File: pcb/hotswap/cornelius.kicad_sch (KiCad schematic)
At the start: 116 parts, among them J1 AVR-ISP-6, SW1 SW_Push, U1 ATmega32U4-M, U2 PRTR5V0U2X, Y1 16MHz

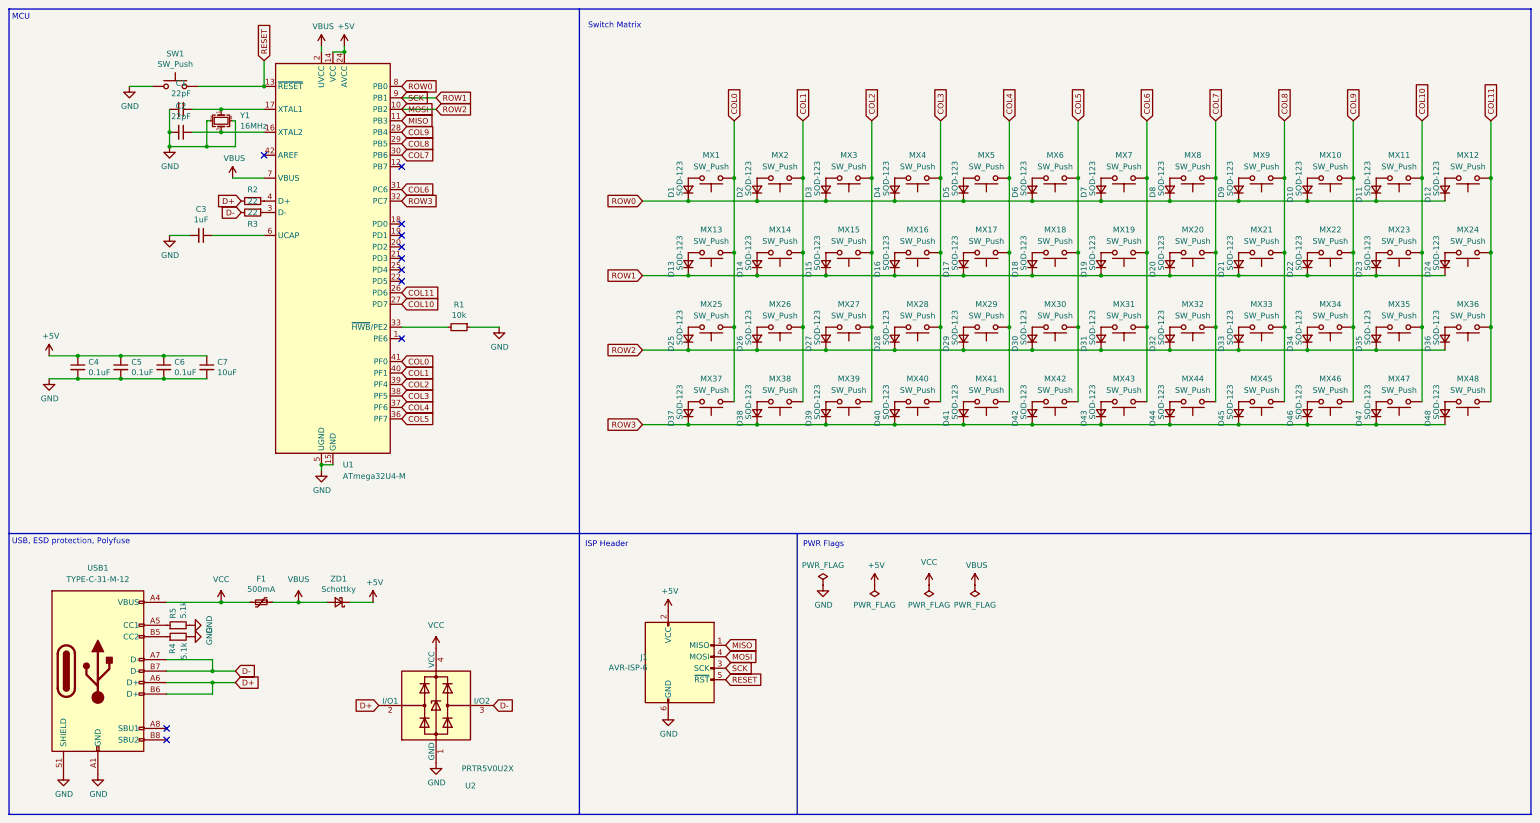
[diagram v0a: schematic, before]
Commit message: Add solder pcb
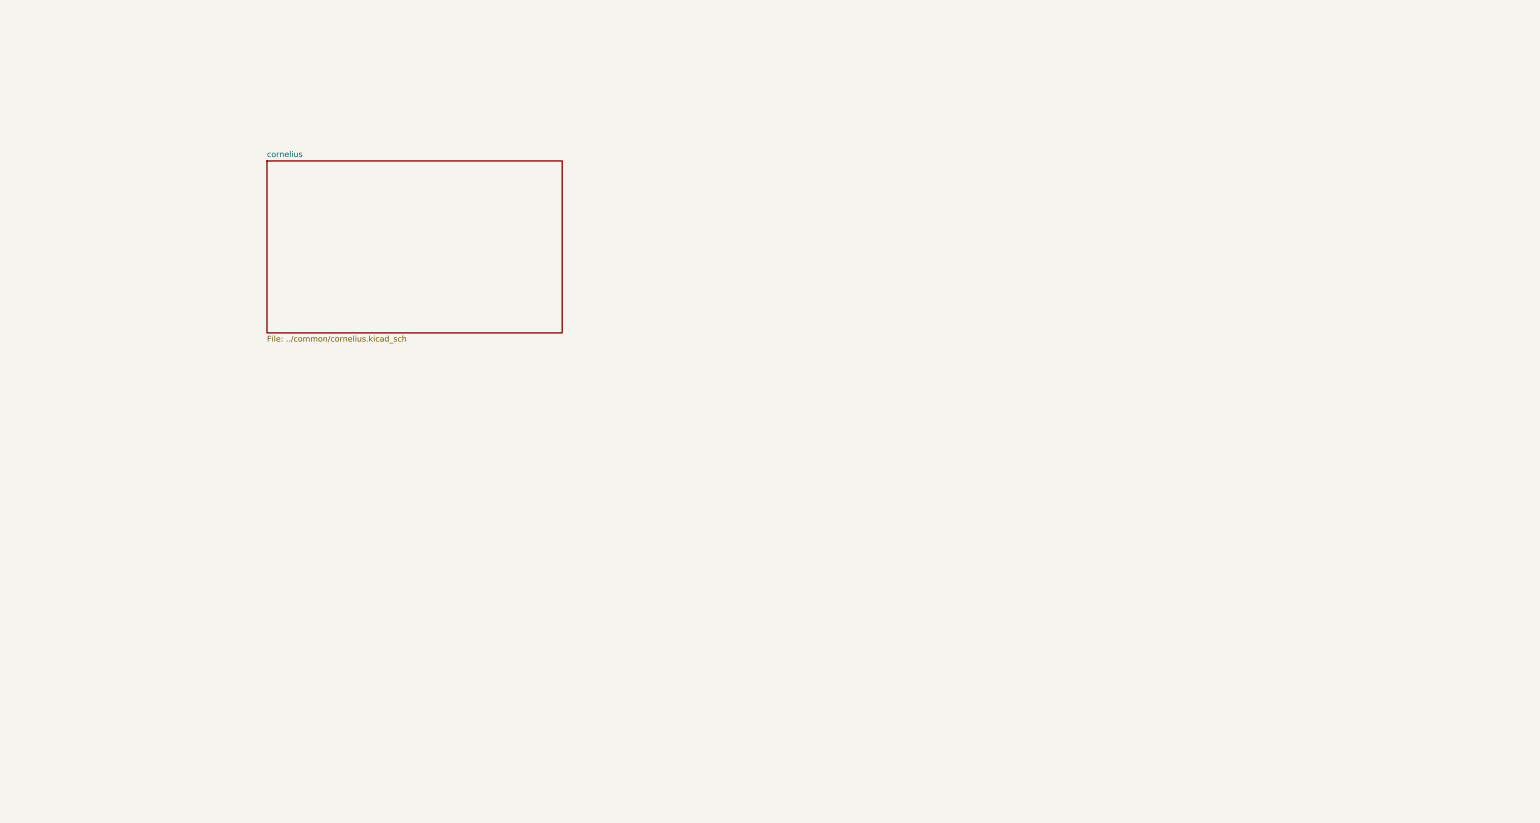
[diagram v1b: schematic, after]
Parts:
- removed C1, C2: 22pF, Capacitor_SMD:C_0603_1608Metric, symbol Device:C_Small
- removed C3: 1uF, Capacitor_SMD:C_0603_1608Metric, symbol Device:C_Small
- removed C4, C5, C6: 0.1uF, Capacitor_SMD:C_0603_1608Metric, symbol Device:C_Small
- removed C7: 10uF, Capacitor_SMD:C_0603_1608Metric, symbol Device:C_Small
- removed D1, D10, D11, D12, D13, D14, D15, D16, D17, D18, D19, D2, D20, D21, D22, D23, D24, D25, D26, D27, D28, D29, D3, D30, D31, D32, D33, D34, D35, D36, D37, D38, D39, D4, D40, D41, D42, D43, D44, D45, D46, D47, D48, D5, D6, D7, D8, D9: SOD-123, Diode_SMD:D_SOD-123, symbol Device:D_Small
- removed F1: 500mA, Fuse:Fuse_1206_3216Metric, symbol Device:Polyfuse_Small
- removed J1: AVR-ISP-6, Connector_PinHeader_2.54mm:PinHeader_2x03_P2.54mm_Vertical, symbol Connector:AVR-ISP-6
- removed MX1, MX10, MX11, MX12, MX13, MX14, MX15, MX16, MX17, MX18, MX19, MX2, MX20, MX21, MX22, MX23, MX24, MX25, MX26, MX27, MX28, MX29, MX3, MX30, MX31, MX32, MX33, MX34, MX35, MX36, MX37, MX38, MX39, MX4, MX40, MX41, MX42, MX43, MX44, MX45, MX46, MX47, MX48, MX5, MX6, MX7, MX8, MX9: SW_Push, kbd:keyswitch_cherrymx_hotswap_1u, symbol Switch:SW_Push
- removed R1: 10k, Resistor_SMD:R_0805_2012Metric, symbol Device:R_Small
- removed R2, R3: 22, Resistor_SMD:R_0805_2012Metric, symbol Device:R_Small
- removed R4, R5: 5.1k, Resistor_SMD:R_0805_2012Metric, symbol Device:R_Small
- removed SW1: SW_Push, Button_Switch_SMD:SW_SPST_SKQG_WithStem, symbol Switch:SW_Push
- removed U1: ATmega32U4-M, Package_DFN_QFN:QFN-44-1EP_7x7mm_P0.5mm_EP5.2x5.2mm, symbol MCU_Microchip_ATmega:ATmega32U4-M
- removed U2: PRTR5V0U2X, Package_TO_SOT_SMD:SOT-143, symbol Power_Protection:PRTR5V0U2X
- removed USB1: TYPE-C-31-M-12, Connector_USB:USB_C_Receptacle_HRO_TYPE-C-31-M-12, symbol Connector:USB_C_Receptacle_USB2.0
- removed Y1: 16MHz, Crystal:Crystal_SMD_3225-4Pin_3.2x2.5mm, symbol Device:Crystal_GND24_Small
- removed ZD1: Schottky, Diode_SMD:D_SOD-123, symbol Device:D_Schottky_Small
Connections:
- no-connect marks 11 -> 0
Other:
- added sheet cornelius (../common/cornelius.kicad_sch)
- note removed: "ISP Header"
- note removed: "MCU"
- note removed: "PWR Flags"
- note removed: "Switch Matrix"
- note removed: "USB, ESD protection, Polyfuse"
